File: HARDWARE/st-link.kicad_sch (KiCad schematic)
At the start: 23 parts, among them J3 USB_B_Micro, Q1 BC848, U5 STM32F103CBTx, U6 LD3985M33R_SOT23, Y2 8 MHz

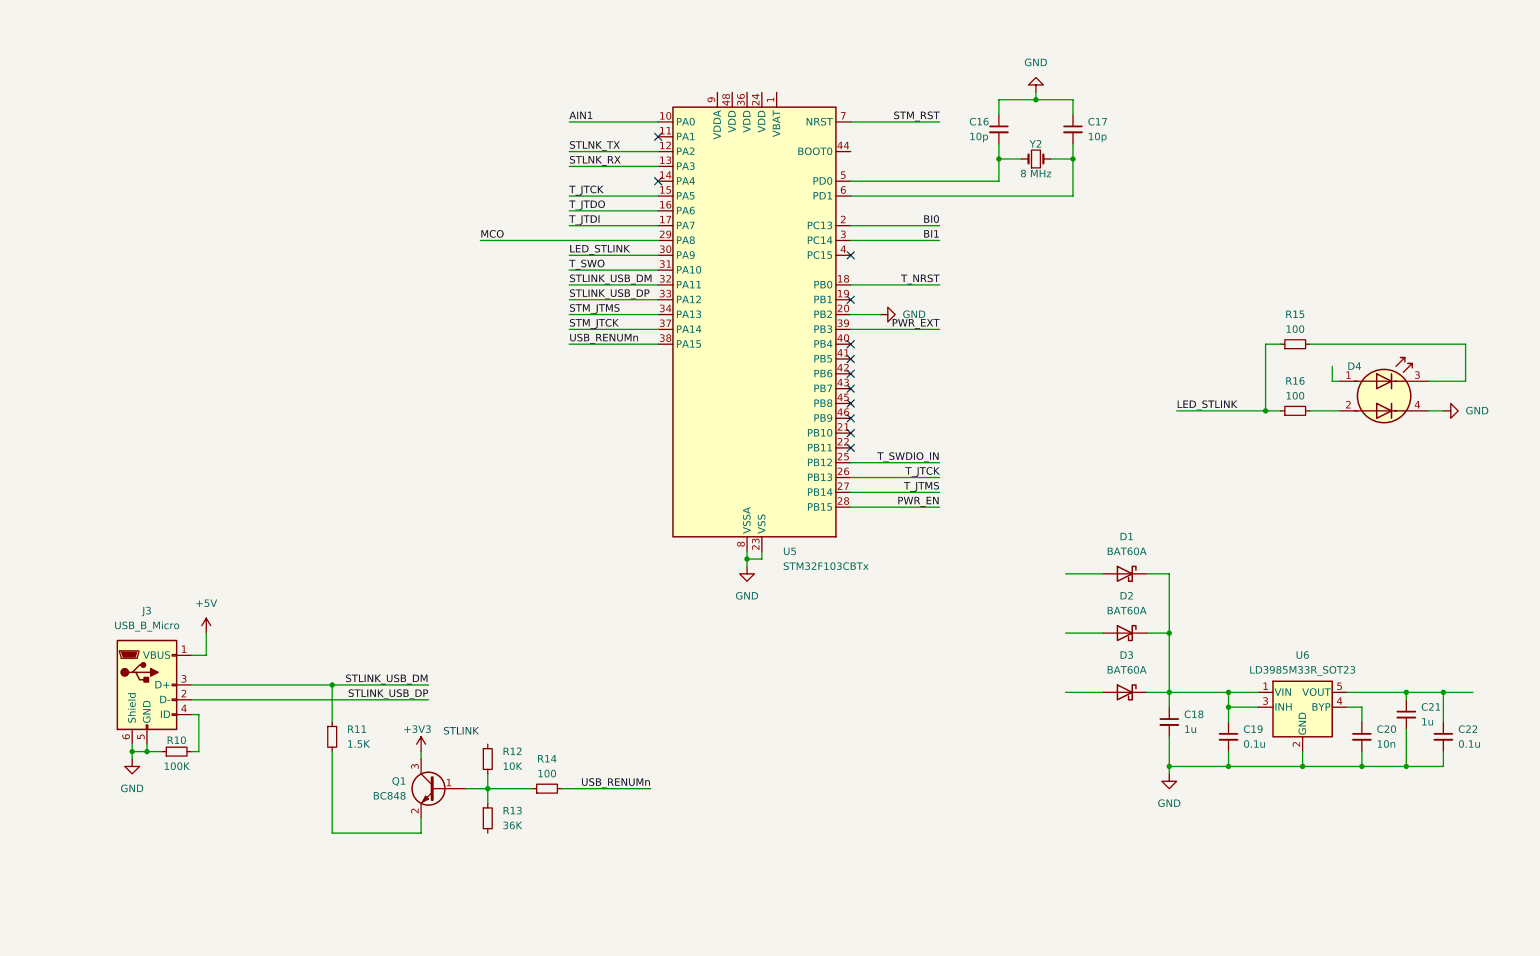
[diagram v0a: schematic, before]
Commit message: schematic capture
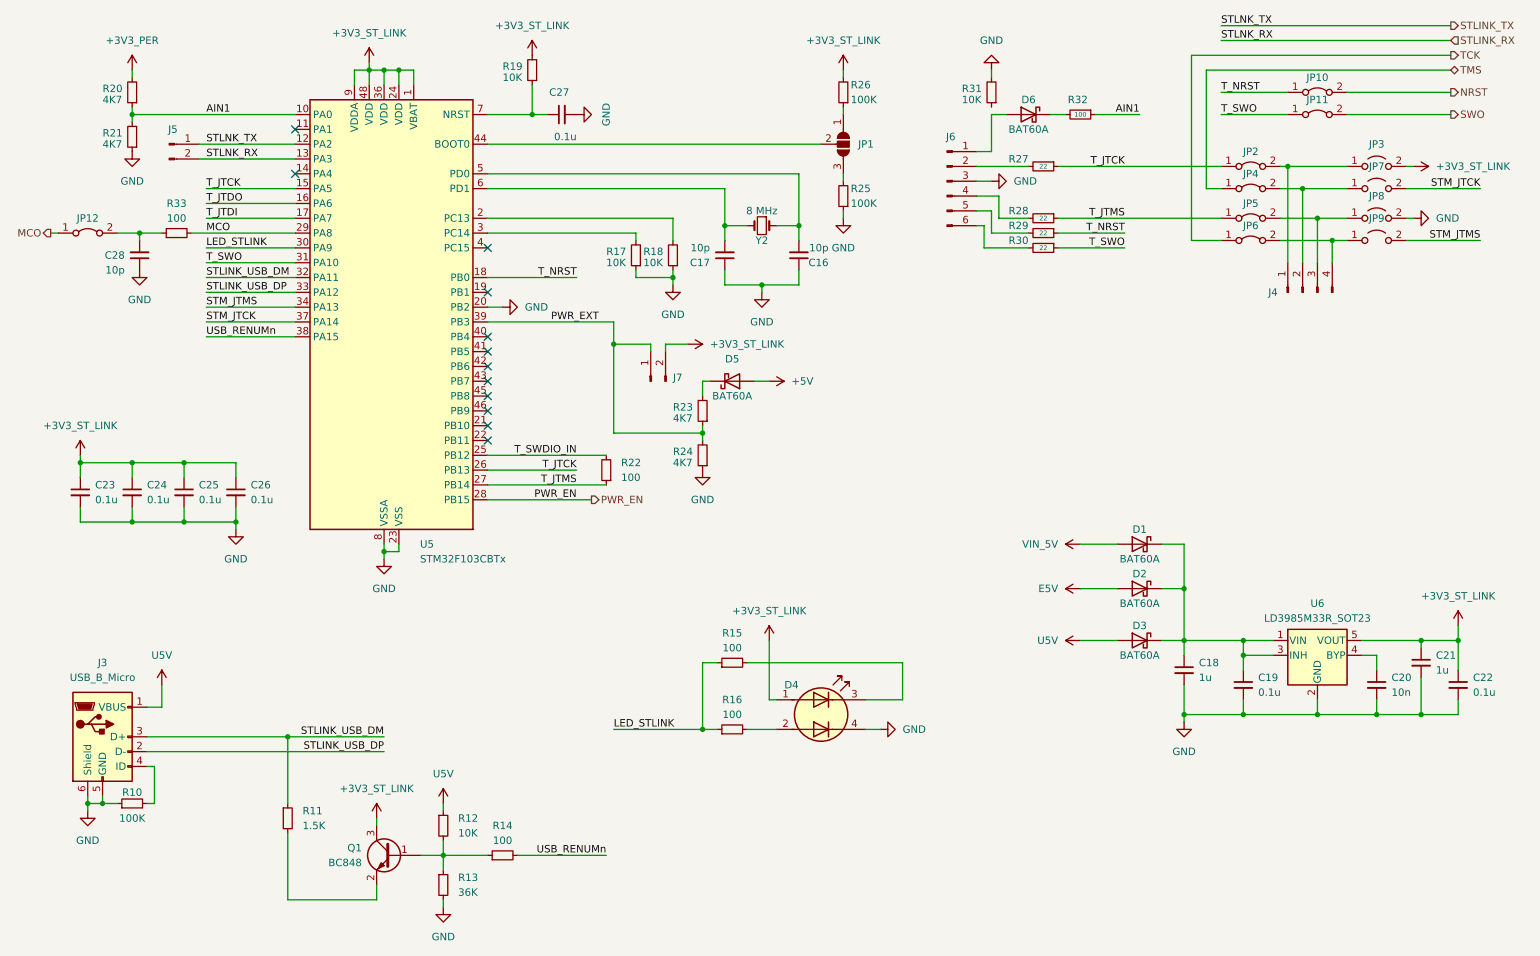
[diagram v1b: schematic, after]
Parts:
- added C23, C24, C25, C26, C27: 0.1u, Resistor_SMD:R_0603_1608Metric, symbol Device:C_Small
- added C28: 10p, symbol Device:C_Small
- added D5, D6: BAT60A, Diode_SMD:D_SOD-323, symbol Diode:BAT60A
- added J4: Conn_01x04_Pin, symbol Connector:Conn_01x04_Pin
- added J5, J7: Conn_01x02_Pin, symbol Connector:Conn_01x02_Pin
- added J6: Conn_01x06_Pin, symbol Connector:Conn_01x06_Pin
- added JP1: SolderJumper_3_Open, symbol Jumper:SolderJumper_3_Open
- added JP10, JP11, JP12, JP2, JP4, JP5, JP6: Jumper_2_Bridged, symbol Jumper:Jumper_2_Bridged
- added JP3, JP7, JP8, JP9: Jumper_2_Open, symbol Jumper:Jumper_2_Open
- added R17, R18, R19, R31: 10K, symbol Device:R_Small
- added R20, R21, R23, R24: 4K7, symbol Device:R_Small
- added R22, R32, R33: 100, symbol Device:R_Small
- added R25, R26: 100K, symbol Device:R_Small
- added R27, R28, R29, R30: 22, symbol Device:R_Small
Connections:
- net +3V3: now also C21.1, C22.1, D4.1 (A1), U5.1 (VBAT), U5.24 (VDD), U5.36 (VDD), U5.48 (VDD), U5.9 (VDDA), U6.5 (VOUT), C23.1, C24.1, C25.1, C26.1, J7.2 (Pin_2), JP3.2 (B), R19.2, R20.2, R26.2
- net +5V: now also D5.2 (A); no longer J3.1 (VBUS)
- net AIN1: now also R20.1, R21.2, R32.1
- net GND: now also R13.2, C23.2, C24.2, C25.2, C26.2, C27.2, C28.1, J6.3 (Pin_3), JP8.2 (B), R17.1, R18.1, R21.1, R24.1, R25.1, R31.2
- net MCO: now also JP12.1 (A), R33.2
- net PWR_EXT: now also J7.1 (Pin_1), R23.1, R24.2
- net STM_JTCK: now also JP7.2 (B)
- net STM_JTMS: now also JP9.2 (B)
- net T_JTCK: now also JP2.1 (A), R27.1
- net T_JTMS: now also JP5.1 (A), R22.1, R28.1
- net T_NRST: now also JP10.1 (A), R29.1
- net T_SWDIO_IN: now also R22.2
- net T_SWO: now also JP11.1 (A), R30.1
- net +5V0: now reaches D2.2 (A)
- net +5V0: now also D1.2 (A), D3.2 (A), J3.1 (VBUS), R12.1
- net at U5.44 (BOOT0): now also JP1.2 (C)
- net BI0: no longer names the net of U5.2 (PC13)
- net BI0: now also R18.2
- net BI1: no longer names the net of U5.3 (PC14)
- net BI1: now also R17.2
- net STLNK_RX renamed STLINK_RX
- net STLINK_RX: now also J5.2 (Pin_2)
- net STLNK_TX renamed STLINK_TX
- net STLINK_TX: now also J5.1 (Pin_1)
- net STM_RST: no longer names the net of U5.7 (NRST)
- net STM_RST: now also C27.1, R19.1
- new net: D6.1 (K), R32.2
- new net: J4.1 (Pin_1), JP2.2 (B), JP3.1 (A)
- new net: J6.6 (Pin_6), R30.2
- new net: C28.2, JP12.2 (B), R33.1
- new net: J6.5 (Pin_5), R29.2
- new net: D6.2 (A), J6.1 (Pin_1)
- new net: JP1.1 (A), R26.1
- new net: J4.2 (Pin_2), JP4.2 (B), JP7.1 (A)
- new net: D5.1 (K), R23.2
- new net: J6.2 (Pin_2), R27.2
- new net: J6.4 (Pin_4), R28.2
- new net: J4.3 (Pin_3), JP5.2 (B), JP8.1 (A)
- new net: JP1.3 (B), R25.2
- new net: J4.4 (Pin_4), JP6.2 (B), JP9.1 (A)
- new net NRST: JP10.2 (B)
- new net SWO: JP11.2 (B)
- new net TCK: JP6.1 (A)
- new net TMS: JP4.1 (A)
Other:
- note removed: "STLINK"
- moved on the sheet: C18, C19, C20, C21, C22, D1, D2, D3, D4, J3, Q1, R10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
